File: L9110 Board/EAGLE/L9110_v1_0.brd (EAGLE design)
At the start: 90 x 90 mm, 46 parts, among them IC5 MCP23017SP, X4 057-016-0

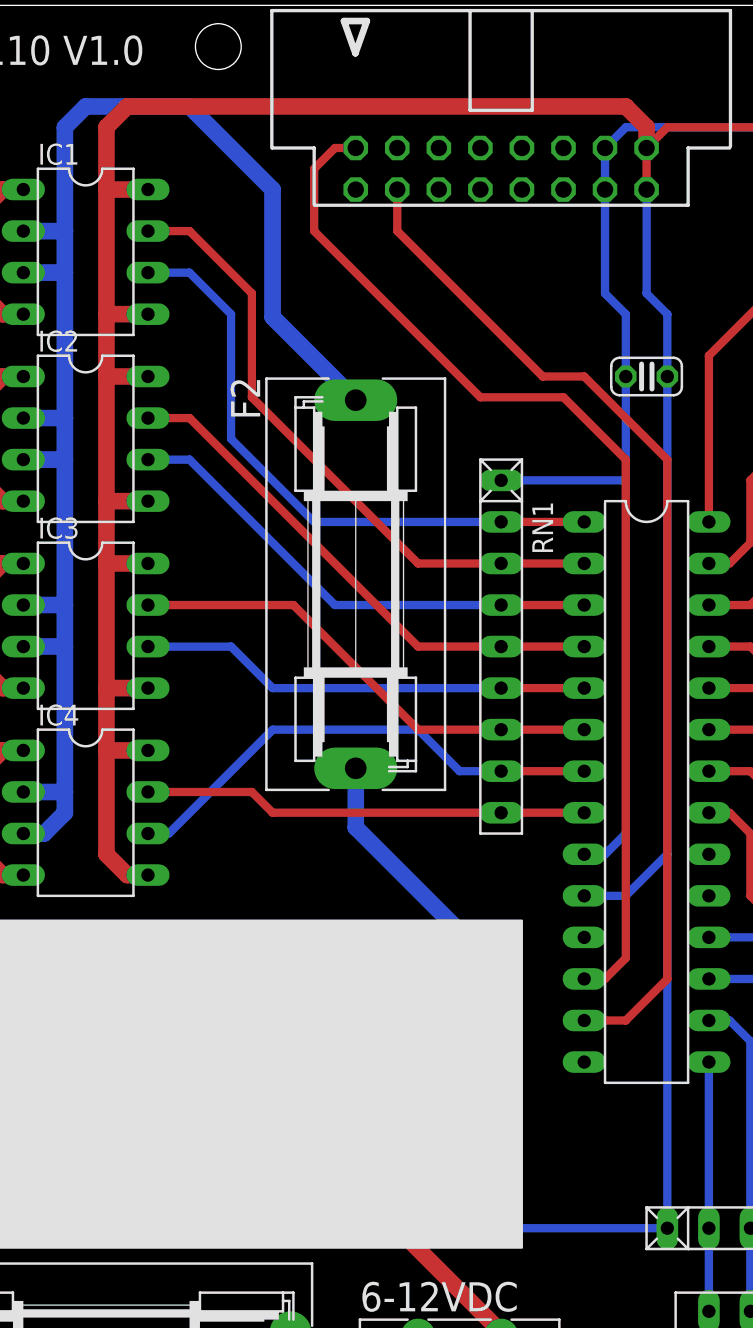
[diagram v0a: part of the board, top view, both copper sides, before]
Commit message: Update L9110_v1_0.brd
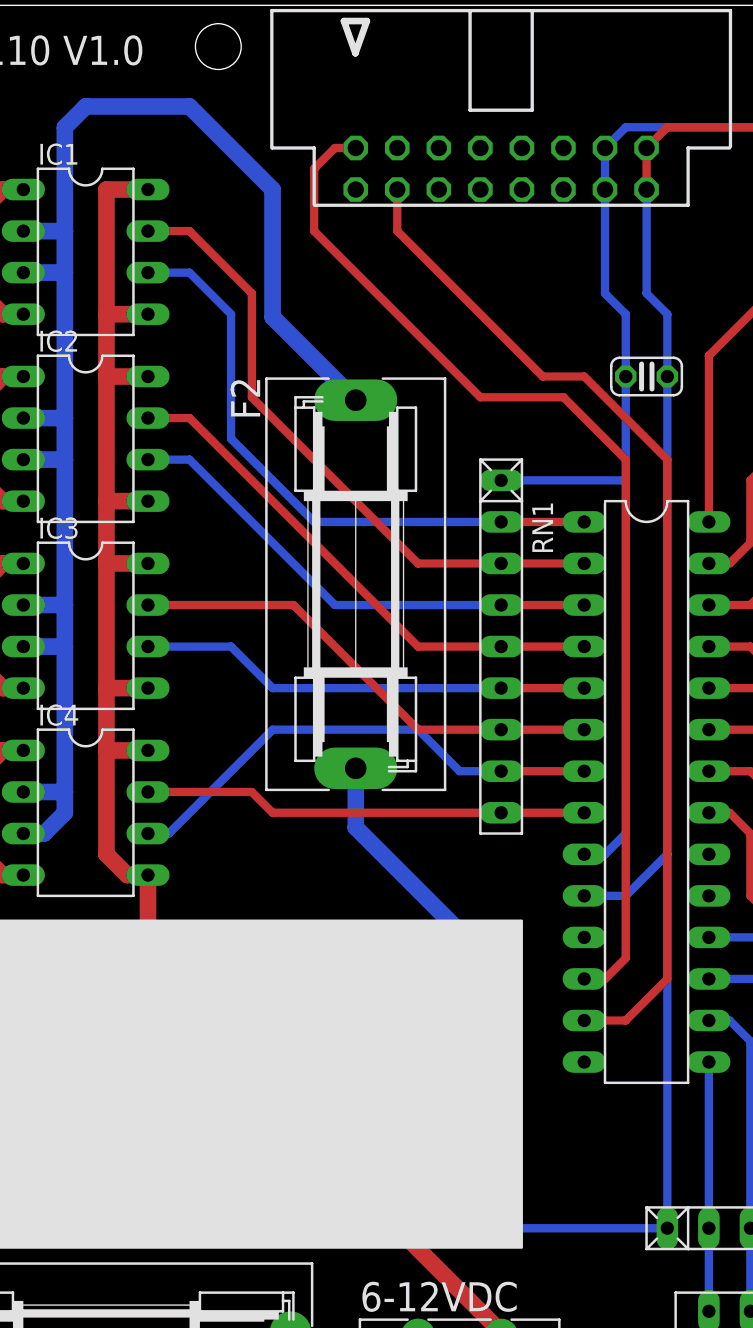
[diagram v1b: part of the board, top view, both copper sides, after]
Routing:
- net GND2: track 308.5 -> 306.3 mm
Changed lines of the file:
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@@
 <wire x1="21.59" y1="67.31" x2="21.59" y2="71.12" width="1.016" layer="1"/>
 <wire x1="21.59" y1="71.12" x2="21.59" y2="78.74" width="1.016" layer="1"/>
-<wire x1="21.59" y1="78.74" x2="21.59" y2="82.55" width="1.016" layer="1"/>
-<wire x1="21.59" y1="82.55" x2="22.86" y2="83.82" width="1.016" layer="1"/>
-<wire x1="53.34" y1="83.82" x2="54.61" y2="82.55" width="1.016" layer="1"/>
-<wire x1="54.61" y1="82.55" x2="54.61" y2="81.28" width="1.016" layer="1"/>
-<wire x1="22.86" y1="83.82" x2="53.34" y2="83.82" width="1.016" layer="1"/>
 <wire x1="24.13" y1="78.74" x2="21.59" y2="78.74" width="1.016" layer="1"/>
 <wire x1="24.13" y1="71.12" x2="21.59" y2="71.12" width="1.016" layer="1"/>
@@
 <wire x1="24.13" y1="48.26" x2="21.59" y2="48.26" width="1.016" layer="1"/>
 <wire x1="24.13" y1="44.45" x2="21.59" y2="44.45" width="1.016" layer="1"/>
+<wire x1="24.13" y1="36.83" x2="24.13" y2="26.67" width="1.016" layer="1"/>
+<wire x1="27.94" y1="22.86" x2="40.64" y2="22.86" width="1.016" layer="1"/>
+<wire x1="40.64" y1="22.86" x2="44.12" y2="19.38" width="1.016" layer="1"/>
+<wire x1="44.12" y1="19.38" x2="44.12" y2="15.65" width="1.016" layer="1"/>
+<wire x1="24.13" y1="26.67" x2="27.94" y2="22.86" width="1.016" layer="1"/>
 </signal>
 <signal name="VCC5.1">

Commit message: Update L9110_v1_0.brd
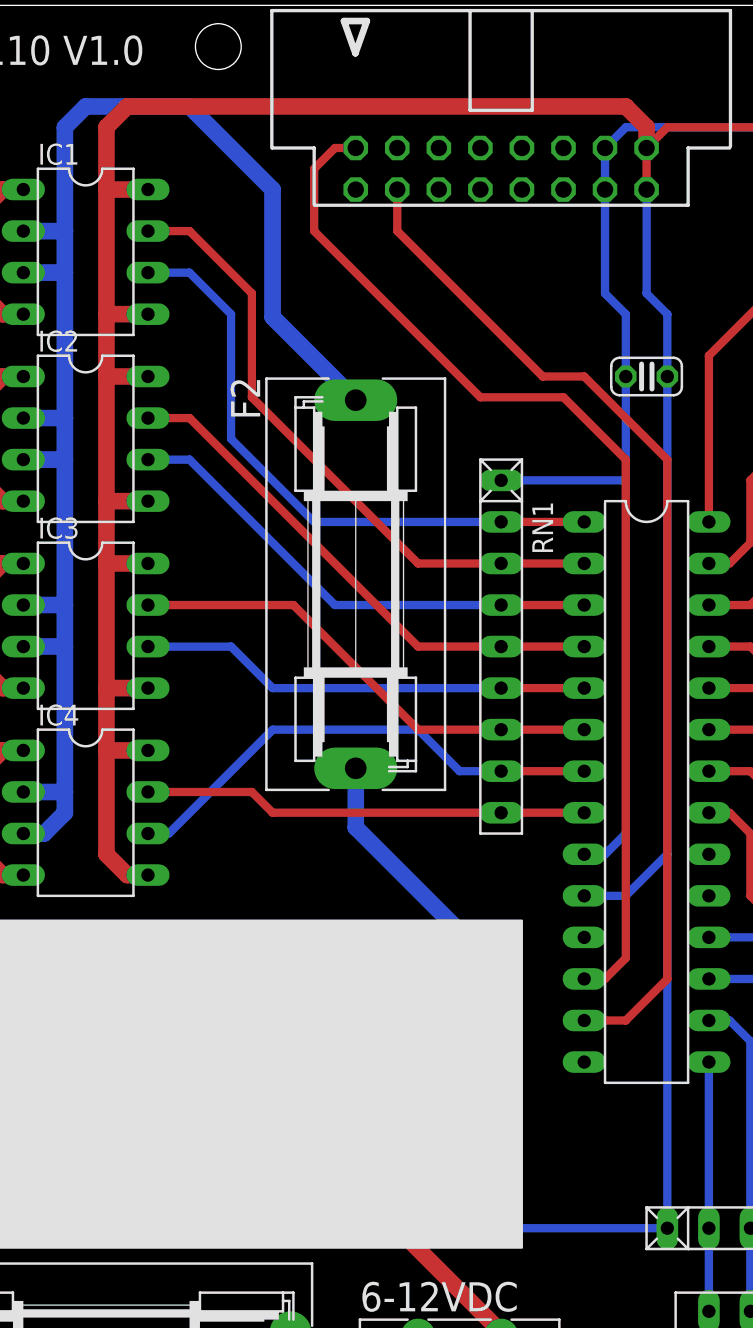
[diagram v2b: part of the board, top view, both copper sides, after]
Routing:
- net GND2: track 306.3 -> 308.5 mm
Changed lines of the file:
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@@
 <wire x1="21.59" y1="67.31" x2="21.59" y2="71.12" width="1.016" layer="1"/>
 <wire x1="21.59" y1="71.12" x2="21.59" y2="78.74" width="1.016" layer="1"/>
+<wire x1="21.59" y1="78.74" x2="21.59" y2="82.55" width="1.016" layer="1"/>
+<wire x1="21.59" y1="82.55" x2="22.86" y2="83.82" width="1.016" layer="1"/>
+<wire x1="53.34" y1="83.82" x2="54.61" y2="82.55" width="1.016" layer="1"/>
+<wire x1="54.61" y1="82.55" x2="54.61" y2="81.28" width="1.016" layer="1"/>
+<wire x1="22.86" y1="83.82" x2="53.34" y2="83.82" width="1.016" layer="1"/>
 <wire x1="24.13" y1="78.74" x2="21.59" y2="78.74" width="1.016" layer="1"/>
 <wire x1="24.13" y1="71.12" x2="21.59" y2="71.12" width="1.016" layer="1"/>
@@
 <wire x1="24.13" y1="48.26" x2="21.59" y2="48.26" width="1.016" layer="1"/>
 <wire x1="24.13" y1="44.45" x2="21.59" y2="44.45" width="1.016" layer="1"/>
-<wire x1="24.13" y1="36.83" x2="24.13" y2="26.67" width="1.016" layer="1"/>
-<wire x1="27.94" y1="22.86" x2="40.64" y2="22.86" width="1.016" layer="1"/>
-<wire x1="40.64" y1="22.86" x2="44.12" y2="19.38" width="1.016" layer="1"/>
-<wire x1="44.12" y1="19.38" x2="44.12" y2="15.65" width="1.016" layer="1"/>
-<wire x1="24.13" y1="26.67" x2="27.94" y2="22.86" width="1.016" layer="1"/>
 </signal>
 <signal name="VCC5.1">
